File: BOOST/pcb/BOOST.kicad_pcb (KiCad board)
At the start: 4 copper layers, 27.9 x 17.8 mm, 25 parts, among them J1 JST, U1 MCP73831-2-OT, U2 TPS61090

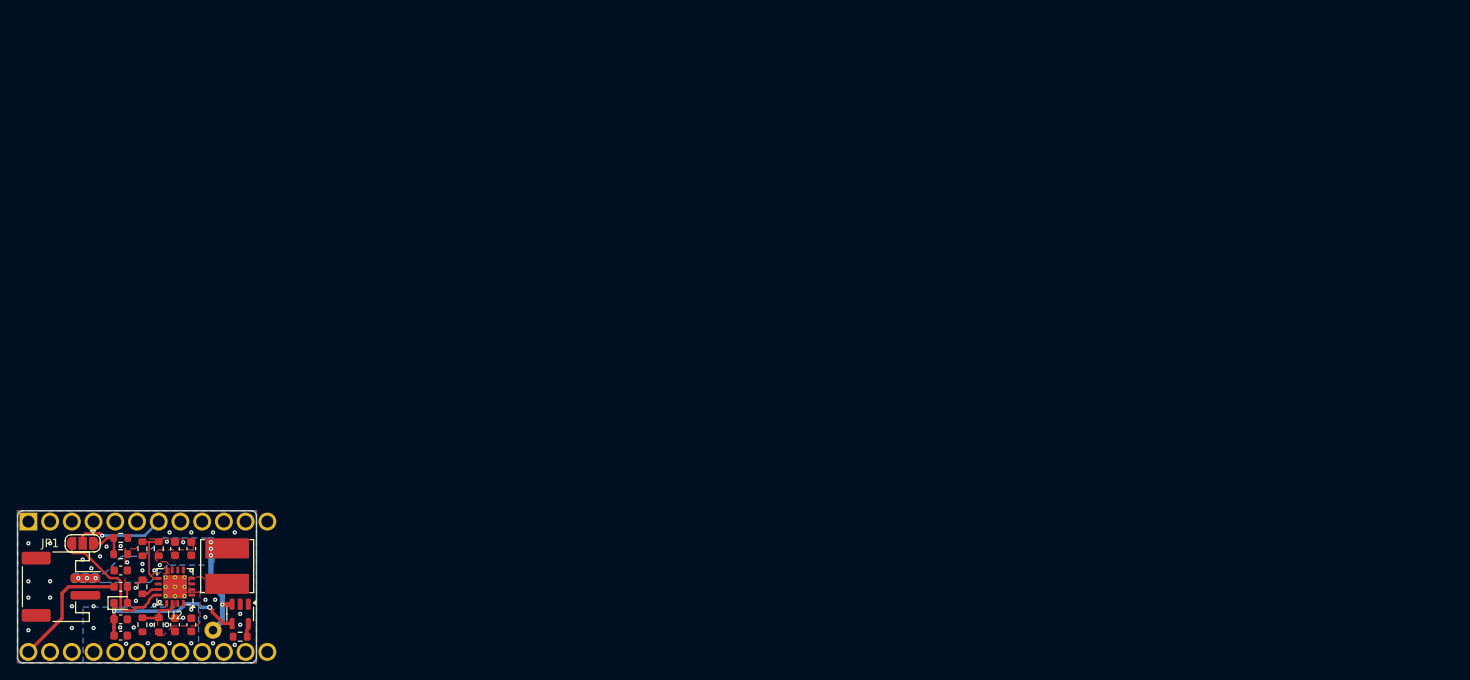
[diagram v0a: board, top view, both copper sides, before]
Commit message: update license
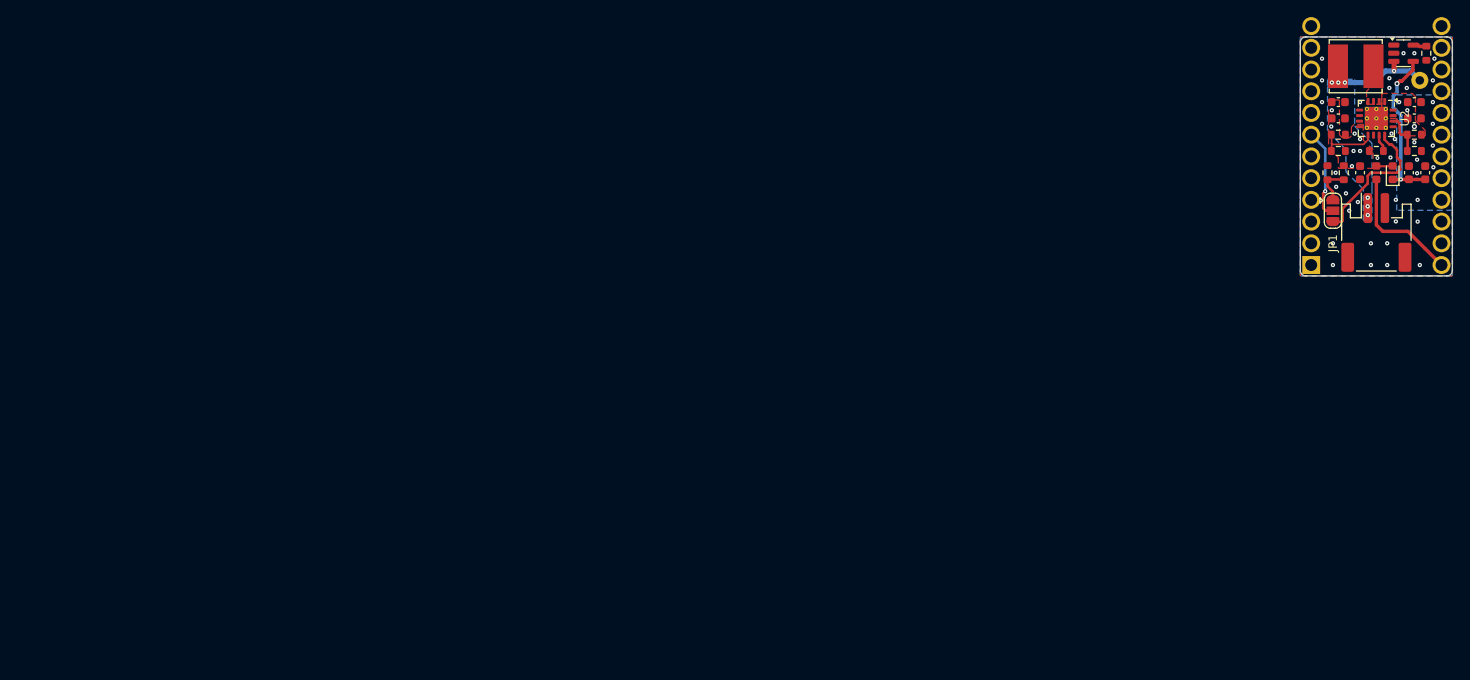
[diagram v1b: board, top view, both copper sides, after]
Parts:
- moved C2 161.9 mm to (226.7, 74.1), turned to -90 degrees
- moved C1 159.4 mm to (224.8, 74.1), turned to 90 degrees
- moved J1 159.3 mm to (221.0, 81.1), turned to 0 degrees
- moved R8 158.7 mm to (225.4, 71.6), turned to 0 degrees
- moved R7 157.6 mm to (225.4, 69.7), turned to 180 degrees
- moved D1 157.0 mm to (222.9, 74.1), turned to 90 degrees
- moved C7 156.5 mm to (225.4, 67.8), turned to 0 degrees
- moved C6 155.5 mm to (225.4, 65.9), turned to 0 degrees
- moved TP1 155.1 mm to (226.1, 63.3), turned to 0 degrees
- moved F1 154.6 mm to (221.0, 74.1), turned to 90 degrees
- moved R3 154.6 mm to (226.8, 60.2), turned to 90 degrees
- moved R4 153.0 mm to (221.0, 71.6), turned to 180 degrees
- moved A1 153.0 mm to (213.4, 84.9), turned to 0 degrees
- moved C5 152.2 mm to (219.1, 74.1), turned to -90 degrees
- moved JP1 151.3 mm to (215.9, 78.6), turned to -90 degrees
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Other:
- board size 27.9 x 17.8 mm -> 17.8 x 27.9 mm
- board text added: "0"
- board text added: "0 mm"
- board text added: "0,01 mm"
- board text added: "0,0152 mm"
- board text added: "0,02"
- board text added: "0,035 mm"
- board text added: "0,1250 mm / 0,0000 mm"
- board text added: "0,2000 mm"
- board text added: "0,2104 mm"
- board text added: "0,25 mm"
- board text added: "0,7912 mm"
- board text added: "1"
- board text added: "17,7800 mm x 27,9400 mm"
- board text added: "3,3"
- board text added: "4"
- board text added: "4,5"
- board text added: "B.Cu"
- board text added: "B.Mask"
- board text added: "B.Paste"
- board text added: "B.Silkscreen"
- board text added: "BOARD CHARACTERISTICS"
- board text added: "Board Thickness:"
- board text added: "Board overall dimensions:"
- board text added: "Bottom Silk Screen"
- board text added: "Bottom Solder Mask"
- board text added: "Bottom Solder Paste"
- board text added: "Castellated pads:"
- board text added: "Color"
- board text added: "Copper Finish:"
- board text added: "Copper Layer Count:"
- board text added: "Dielectric"
- board text added: "Edge card connectors:"
- board text added: "Epsilon R"
- board text added: "F.Cu"
- board text added: "F.Mask"
- board text added: "F.Paste"
- board text added: "F.Silkscreen"
- board text added: "FR4"
- board text added: "Impedance Control:"
- board text added: "In1.Cu"
- board text added: "In2.Cu"
- board text added: "Layer Name"
- board text added: "Loss Tangent"
- board text added: "Material"
- board text added: "Min hole diameter:"
- board text added: "Min track/spacing:"
- board text added: "No"
- board text added: "None"
- board text added: "Not specified"
- board text added: "Plated Board Edge:"
- board text added: "Thickness (mm)"
- board text added: "Top Silk Screen"
- board text added: "Top Solder Mask"
- board text added: "Top Solder Paste"
- board text added: "Type"
- board text added: "Yes"
- board text added: "copper"
- board text added: "core"
- board text added: "prepreg"
